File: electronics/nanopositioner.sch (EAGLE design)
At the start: 48 parts, among them J1 629722000214, U1 TPS73633DBVR, U2 USBLC6-2SC6, U3 DAC80504RTER, U4 ESP32-S3-WROOM-1-N4R8, U5 LM5157RTERQFN_57RTER_TEX-L

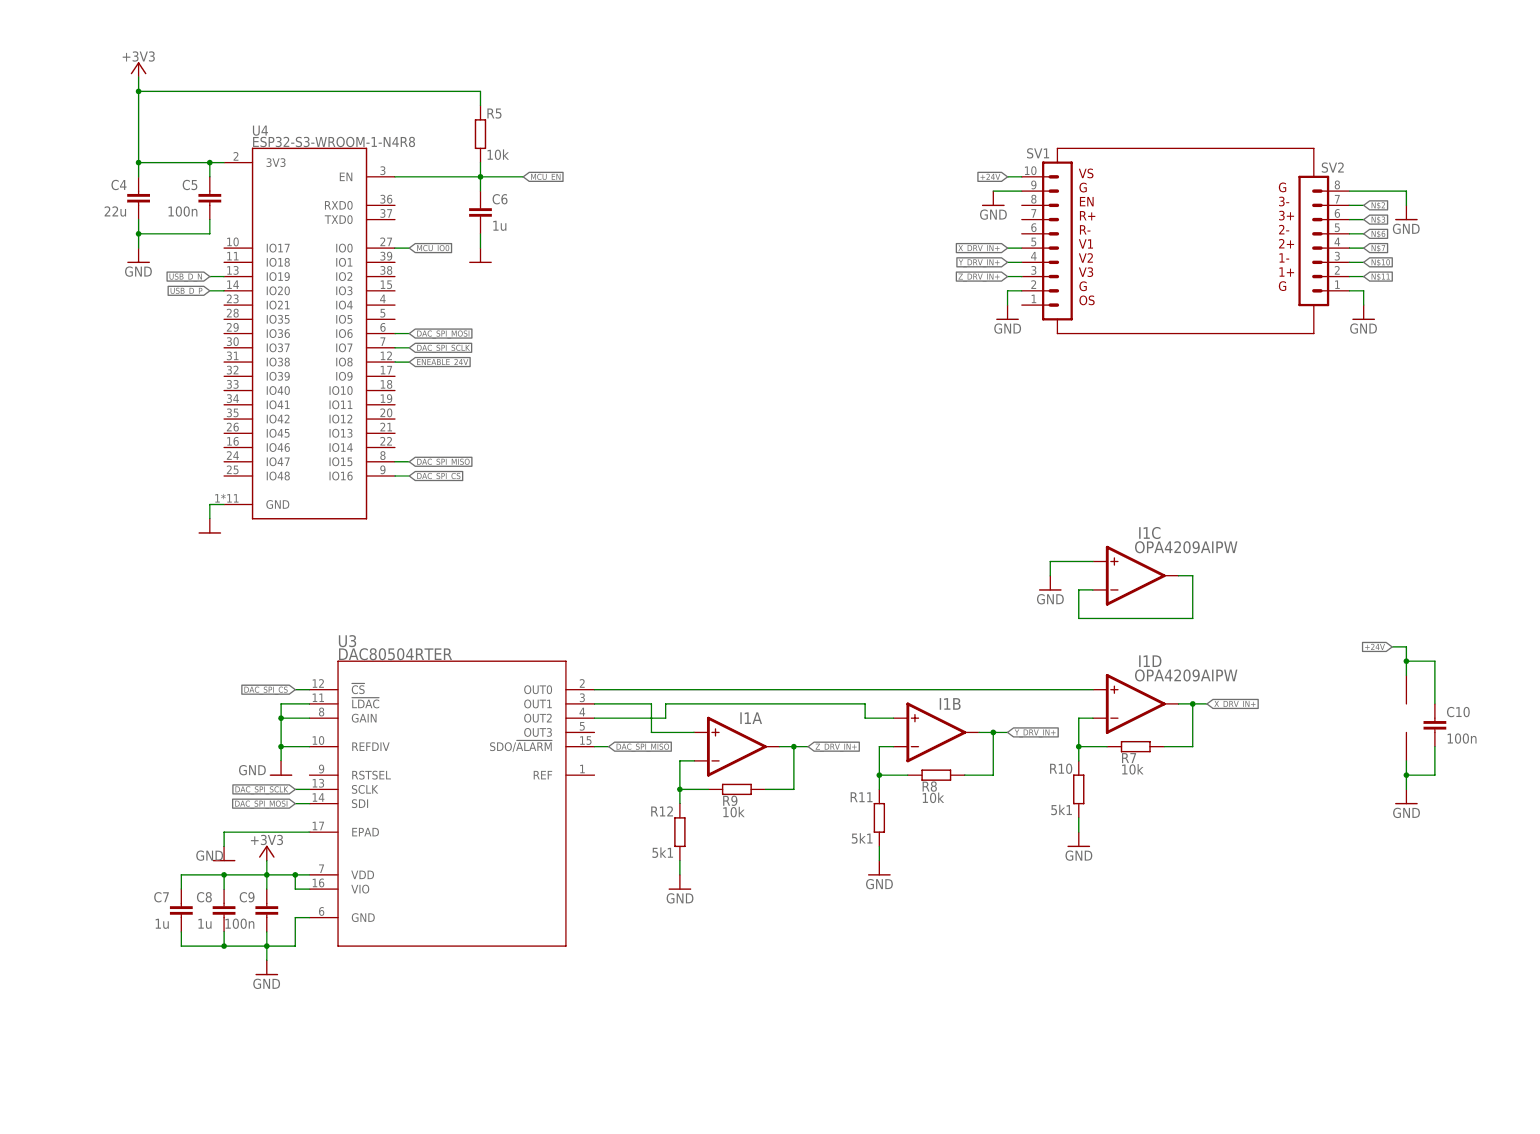
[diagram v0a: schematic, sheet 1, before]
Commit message: a
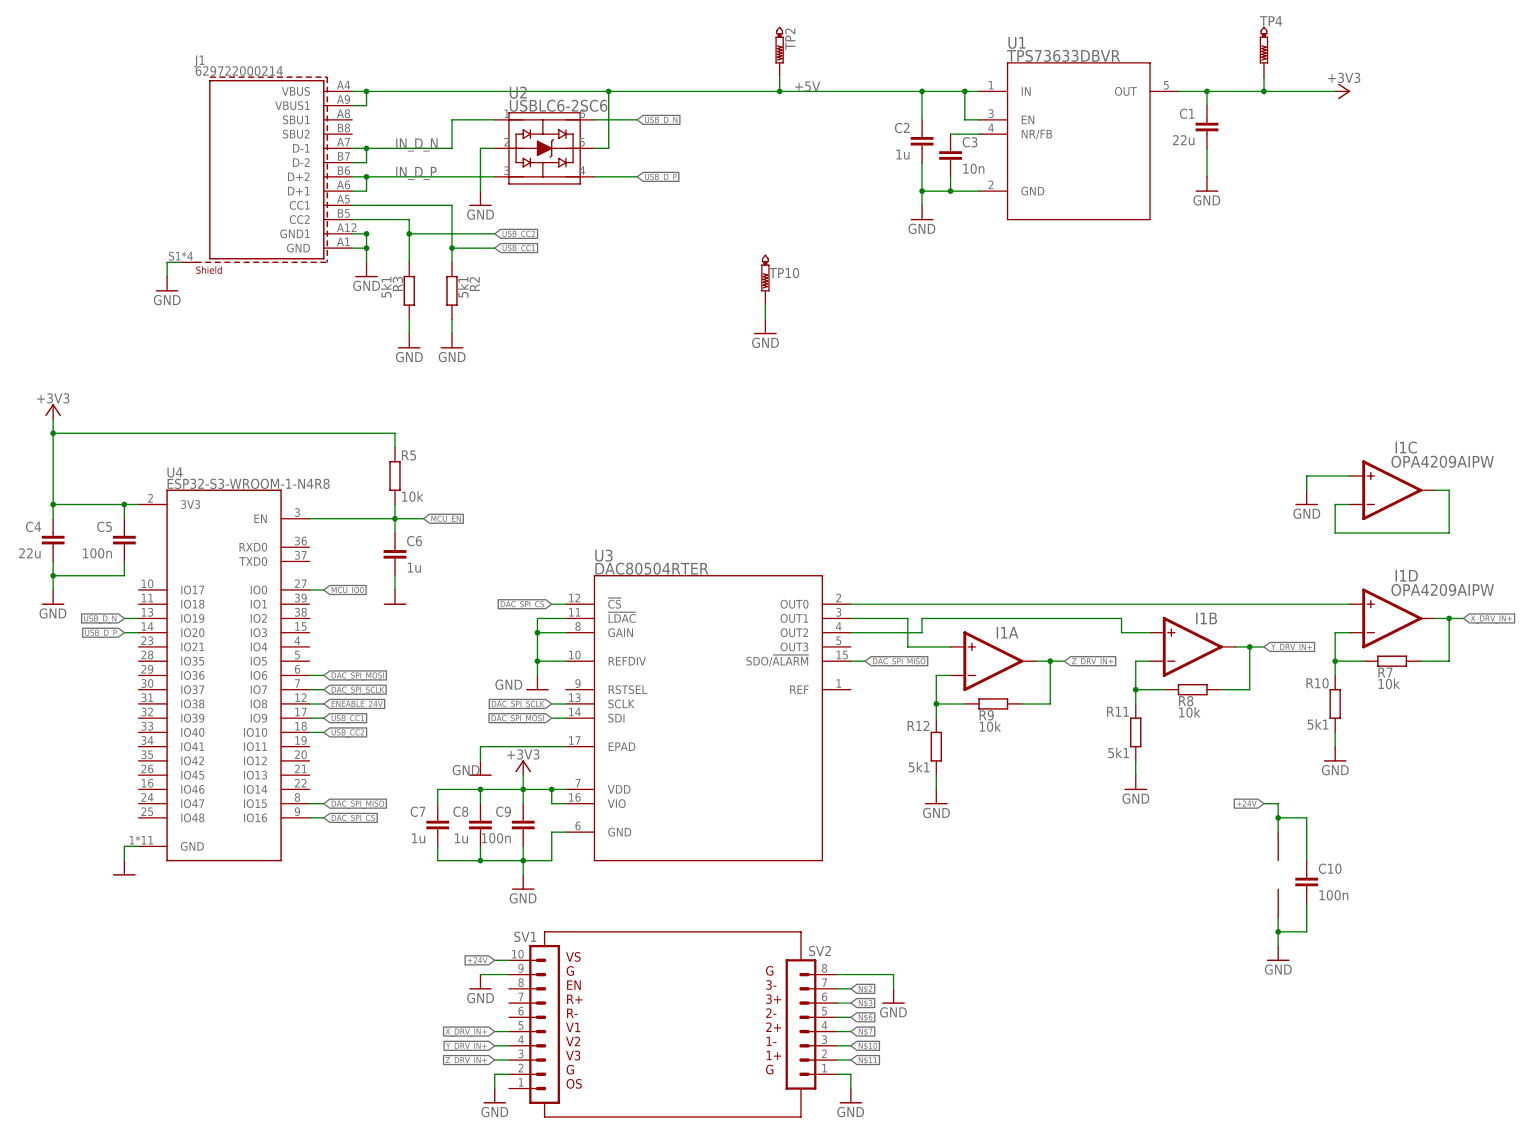
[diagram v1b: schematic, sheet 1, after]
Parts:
- removed TP1: PTR1PAD1-13, testpad:PTR1PAD1-13
- added R6: 57k6, rcl:R-EU_R0402
- C11: value 12n -> 27n
- C12: value 22p -> 5p6
- C14: value 10u -> 6u8; device rcl:C-EUC0402 -> rcl:C-EUC1206
- C15, C16: device rcl:C-EUC0402 -> rcl:C-EUC0603
- C18: value 2u2 -> 6u8; device rcl:C-EUC0402 -> rcl:C-EUC1206
- C19: value 22u -> 6u8; device rcl:C-EUC0603 -> rcl:C-EUC1206
- C20: value 22u -> 2u2; device rcl:C-EUC0603 -> rcl:C-EUC0805
- L1: value 2.7u, 8m -> 2u7, 8m
- R1: value 9k76 -> 1k91
- R13: value 57k6 -> 2k49
- R14: value 2k49 -> 9k76
- R4: value 845r -> 9k76
- U5: value LM5157RTERQFN_57RTER_TEX-L -> LM5157RTER; device dkjdaksndkja:LM5157RTERQFN_57RTER_TEX-L -> dkjdaksndkja:LM5157RTER
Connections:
- removed net N$22 (its old number): R1.2, U5.MODE
- removed net N$24: R13.1, R14.2, U5.FB
- removed net N$27: C17.1, U5.VCC
- removed net N$4: J1.CC1, R2.2
- removed net N$5: J1.CC2, R3.1
- new net N$26: C17.2, U5.VCC
- new net N$8: C11.2, C12.2, U5.COMP
- new net USB_CC1: J1.CC1, R2.2, U4.IO9
- new net USB_CC2: J1.CC2, R3.1, U4.IO10
- net +24V: now also C14.2, C15.2, C18.2, C19.2, R6.1; no longer C14.1, C15.1, C19.1, C20.1, R13.2, TP1.TP
- net +5V: now also C16.2, C20.2; no longer C16.1, C18.1, U5.EN/UVLO/SYNC
- net ENEABLE_24V: now also R14.1, U5.EN/UVLO/SYNC
- net GND: now also C12.1, C13.1, C14.1, C15.1, C16.1, C17.1, C18.1, C19.1, C20.1, R1.2, R13.2, R14.2, R4.2, U5.MODE; no longer C12.2, C13.2, C14.2, C15.2, C16.2, C17.2, C18.2, C19.2, C20.2, R1.1, R14.1, R4.1
- net N$18: now also R1.1; no longer U5.COMP
- net N$20: now also C13.2; no longer C12.1
- net N$21: now also R4.1; no longer C13.1
- net N$23: now also R13.1, R6.2, U5.FB; no longer C11.2, R4.2
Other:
- note added: "+24V"
- note removed: "24V"
- moved on the sheet: C10, C11, C12, C13, C14, C15, C16, C17, C18, C19, C20, C4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

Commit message: fix
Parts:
- C1, C4: MPN (none) -> CL10A226MP8NUNE
- C10, C5, C9: MPN (none) -> GRM155R71H104KE14D
- C11: MPN (none) -> GRM155R71A273KA01D
- C12: MPN (none) -> GRM1555C1H5R6CA01D
- C13: MPN (none) -> GRM033R70J103KA01D
- C14, C18, C19: MPN (none) -> C3216X5R1H685K160AB
- C15: MPN (none) -> CGA3E2X7R1H104K080AA
- C16: MPN (none) -> KGM21NR71E104KT
- C17: MPN (none) -> EMK107B7105KA-T
- C2, C6, C7, C8: MPN (none) -> GRM155R61E105MA12D
- C20: MPN (none) -> GRM21BR71A225KA01L
- C3: MPN (none) -> GCM155R71H103KA55D
- D1: MPN (none) -> B240A-13-F
- I1: MPN (none) -> OPA4209AIPW
- J1: MPN (none) -> 12402012E212A
- L1: MPN (none) -> SDR1307-2R7ML
- R1: MPN (none) -> CRCW04021K91FKED
- R10, R11, R12, R2, R3: MPN (none) -> ERA-2AEB512X
- R13: MPN (none) -> CRCW04022K49FKED
- R14, R4: MPN (none) -> CRCW04029K76FKED
- R5, R7, R8, R9: MPN (none) -> ERA-2AEB103X
- R6: MPN (none) -> CRCW040257K6FKED
- U1: MPN (none) -> TPS73633DBVR
- U2: MPN (none) -> USBLC6-2SC6
- U3: MPN (none) -> DAC80504RTET
- U4: MPN (none) -> ESP32-S3-WROOM-1-N4
- U5: MPN (none) -> LM5157RTER
